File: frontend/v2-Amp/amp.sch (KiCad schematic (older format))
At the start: 72 parts, among them K1 HK4100, P1 Antenna, P2 CONN_02X07, P3 TX Power Tap, P4 TX-IN, P5 RX IN, P6 12-13.8v, Q1 PZT2222A, Q2 RD16HHF1, T1 OUT_TRANSF, T2 BN-43-2402, U1 LP2951-50D

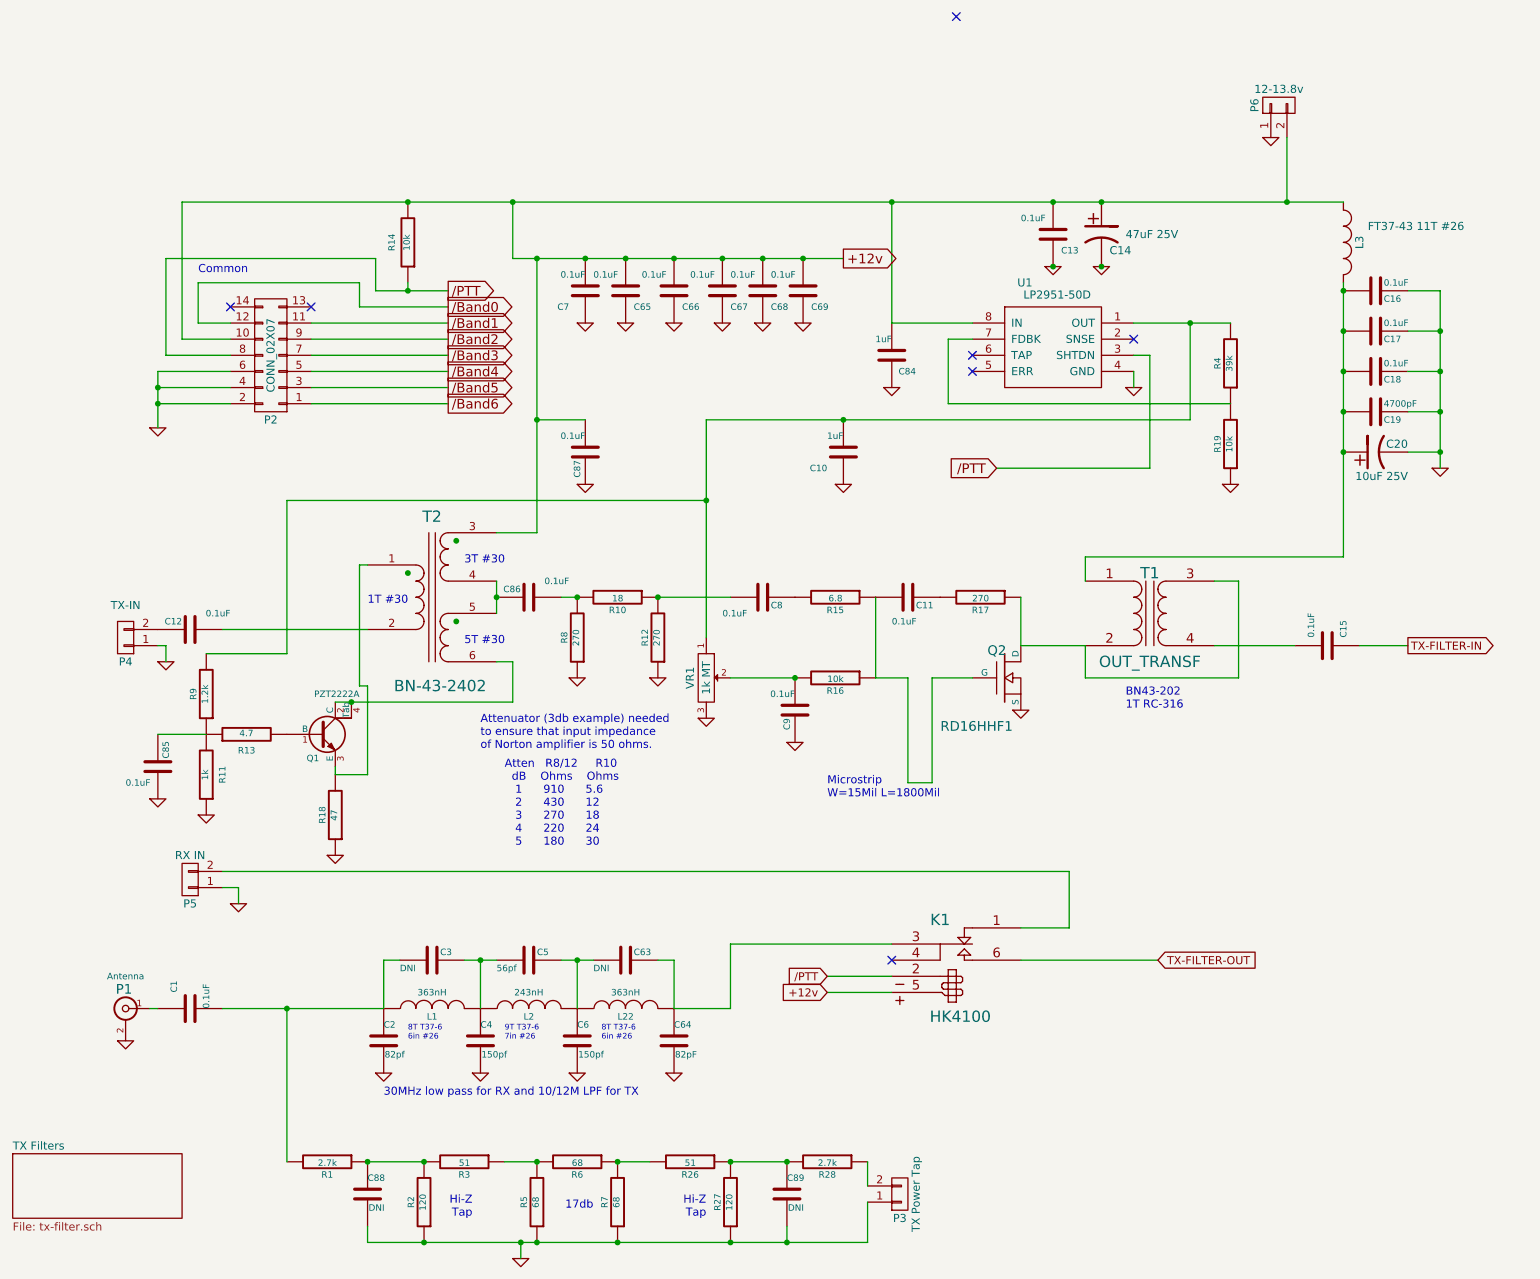
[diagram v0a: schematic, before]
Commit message: Ver 1.1 changes
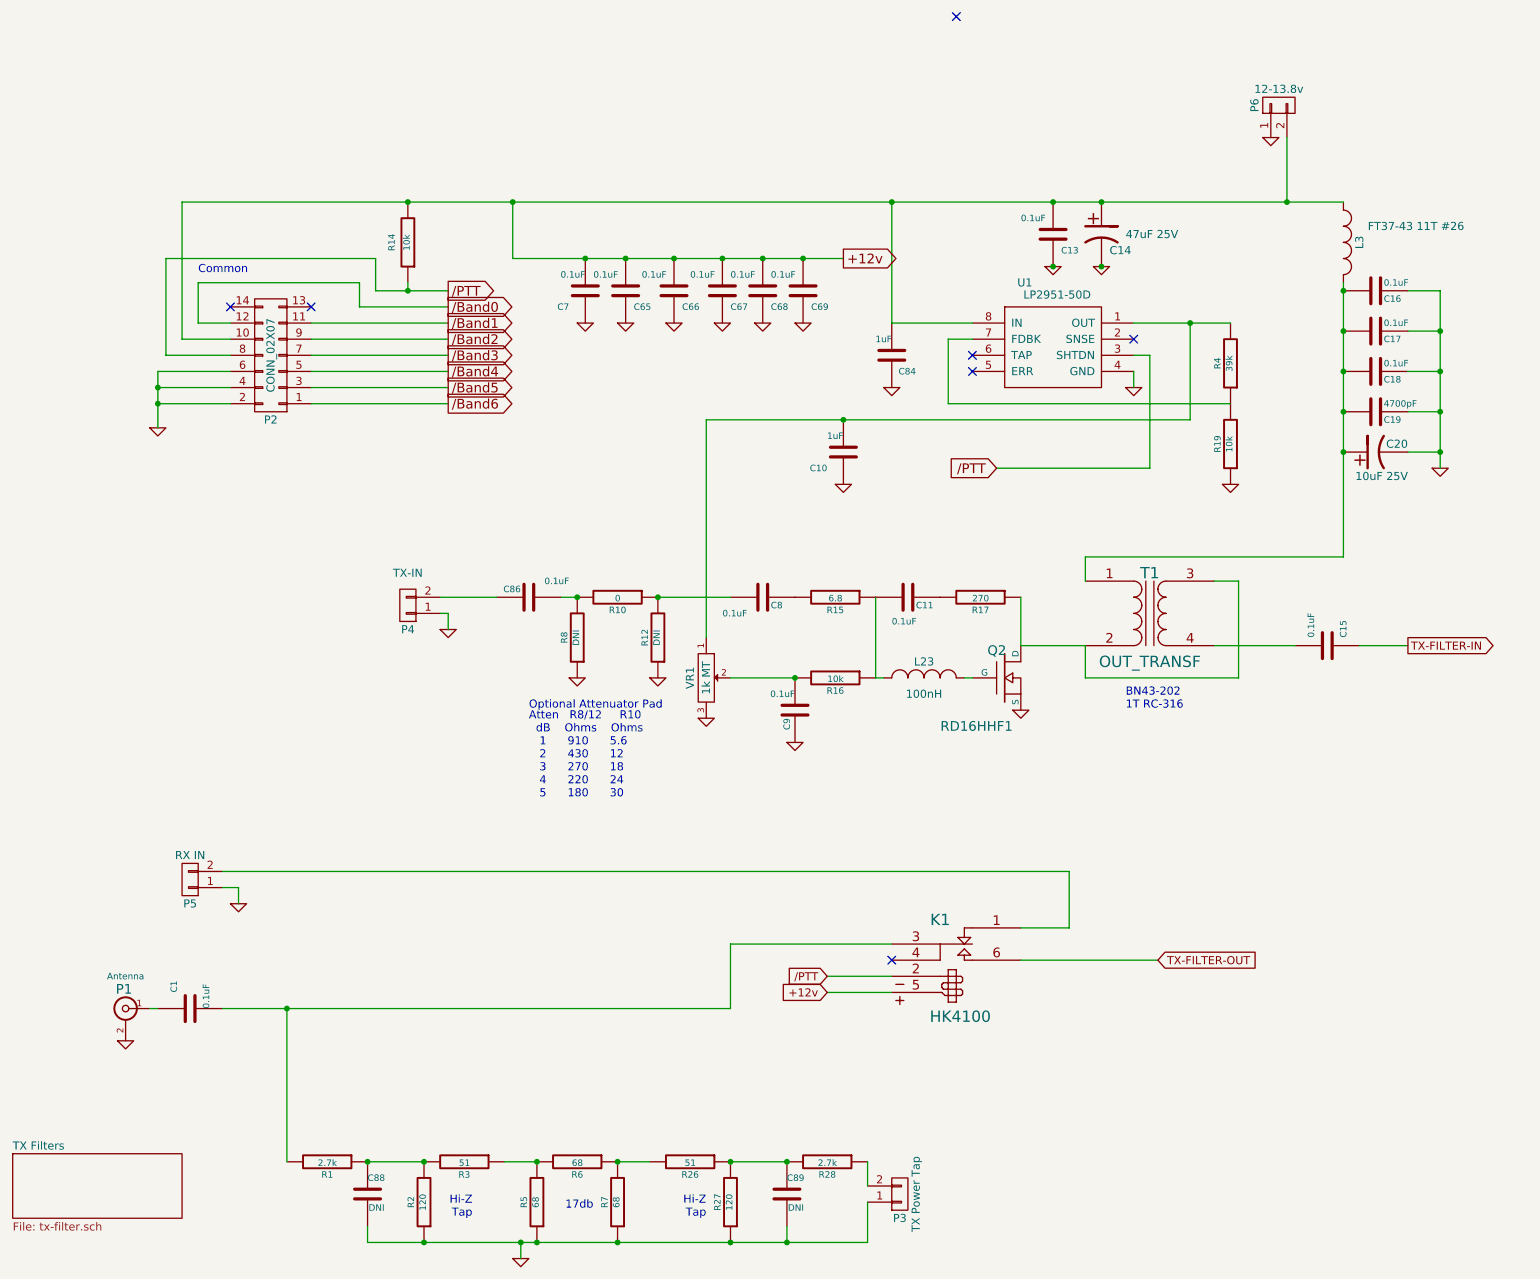
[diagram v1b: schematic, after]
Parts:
- removed C12, C85, C87: 0.1uF, HERMESLITE:C_0805, symbol C-RESCUE-amp
- removed C2: 82pf, HERMESLITE:C_0805, symbol C-RESCUE-amp
- removed C3, C63: DNI, HERMESLITE:C_0805, symbol C-RESCUE-amp
- removed C4, C6: 150pf, HERMESLITE:C_0805, symbol C-RESCUE-amp
- removed C5: 56pf, HERMESLITE:C_0805, symbol C-RESCUE-amp
- removed C64: 82pF, HERMESLITE:C_0805, symbol C-RESCUE-amp
- removed L1, L22: 363nH, HERMESLITE:Choke_Toroid, symbol INDUCTOR
- removed L2: 243nH, HERMESLITE:Choke_Toroid, symbol INDUCTOR
- removed Q1: PZT2222A, TO_SOT_Packages_SMD:SOT-223, symbol PZT2222A-T
- removed R11: 1k, Resistors_SMD:R_0805_HandSoldering, symbol R-RESCUE-amp
- removed R13: 4.7, Resistors_SMD:R_0805_HandSoldering, symbol R-RESCUE-amp
- removed R18: 47, Resistors_SMD:R_0805_HandSoldering, symbol R-RESCUE-amp
- removed R9: 1.2k, Resistors_SMD:R_0805_HandSoldering, symbol R-RESCUE-amp
- removed T2: BN-43-2402, HERMESLITE:TRANSF, symbol TRANSFO2
- added L23: 100nH, Resistors_SMD:R_0805_HandSoldering, symbol INDUCTOR_SMALL
- Q2: footprint Transistors_TO-220:TO-220_Neutral123_Vertical -> TO_SOT_Packages_THT:TO-220_Neutral123_Vertical
- R10: value 18 -> 0
- R12, R8: value 270 -> DNI
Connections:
- net at C11.2, R15.1, R16.1: now also L23.1; no longer Q2.1 (G)
- net at C1.2, R1.2: now also K1.3
- net at P4.2 (P2): now also C86.1
- new net: L23.2, Q2.1 (G)
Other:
- note added: "Optional Attenuator Pad\n"
- note removed: "1T #30\n"
- note removed: "30MHz low pass for RX and 10/12M LPF for TX"
- note removed: "3T #30\n"
- note removed: "5T #30\n"
- note removed: "8T T37-6\n6in #26"
- note removed: "9T T37-6\n7in #26"
- note removed: "Attenuator (3db example) needed \nto ensure that input impedance\nof Norton amplifier is 50 ohms."
- note removed: "Microstrip\nW=15Mil L=1800Mil"
- moved on the sheet: P4

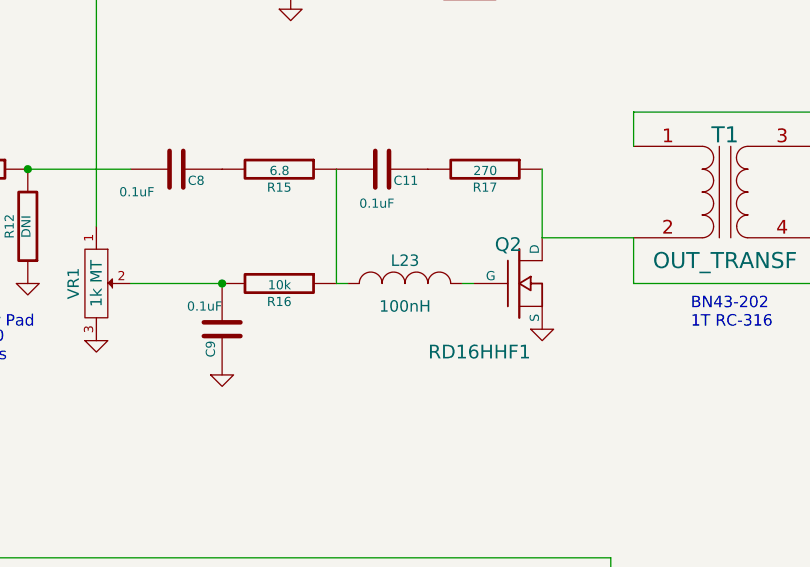
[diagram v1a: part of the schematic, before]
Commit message: Updates for v1.1
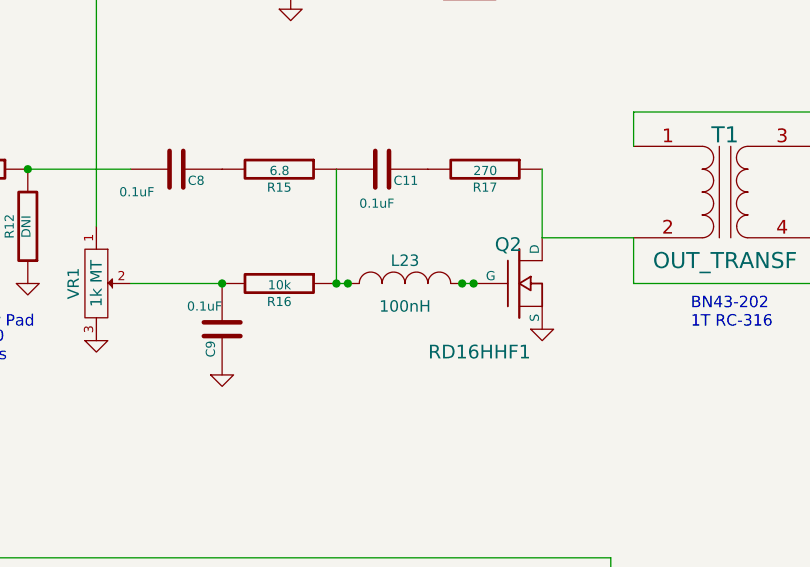
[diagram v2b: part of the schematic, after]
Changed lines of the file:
@@
 Wire Wire Line
 	6450 4200 6500 4200
+Connection ~ 6450 4200
+Connection ~ 6500 4200
+Connection ~ 5950 4200
+Connection ~ 5900 4200
 $EndSCHEMATC
